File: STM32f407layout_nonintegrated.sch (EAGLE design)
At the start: 45 parts, among them Q1 ASF, T3 FDN340P, T4 AP1117_LIN_REG

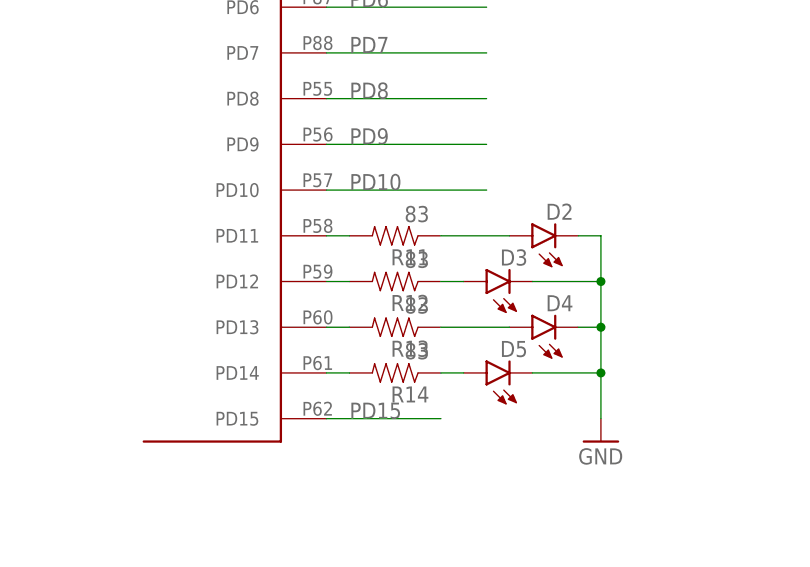
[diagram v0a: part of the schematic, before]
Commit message: Fixed some wrong info
fixed some stuff
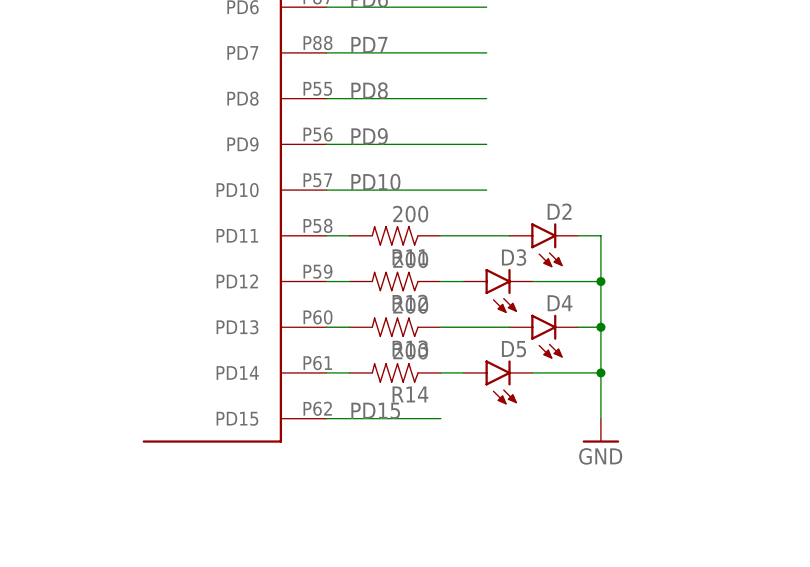
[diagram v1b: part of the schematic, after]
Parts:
- R11, R12, R13, R14: value 83 -> 200
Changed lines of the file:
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@@
 <part name="+3V10" library="supply1" deviceset="+3V3" device=""/>
 <part name="C3" library="SparkFun-Passives" deviceset="CAP" device="0603-CAP" value="0.22uF"/>
-<part name="R11" library="SparkFun-Passives" deviceset="RESISTOR" device="0603-RES" value="83"/>
-<part name="R12" library="SparkFun-Passives" deviceset="RESISTOR" device="0603-RES" value="83"/>
-<part name="R13" library="SparkFun-Passives" deviceset="RESISTOR" device="0603-RES" value="83"/>
-<part name="R14" library="SparkFun-Passives" deviceset="RESISTOR" device="0603-RES" value="83"/>
+<part name="R11" library="SparkFun-Passives" deviceset="RESISTOR" device="0603-RES" value="200"/>
+<part name="R12" library="SparkFun-Passives" deviceset="RESISTOR" device="0603-RES" value="200"/>
+<part name="R13" library="SparkFun-Passives" deviceset="RESISTOR" device="0603-RES" value="200"/>
+<part name="R14" library="SparkFun-Passives" deviceset="RESISTOR" device="0603-RES" value="200"/>
 <part name="C8" library="SparkFun-Passives" deviceset="CAP" device="0603-CAP" value="4.7uF"/>
 <part name="GND15" library="supply1" deviceset="GND" device=""/>
